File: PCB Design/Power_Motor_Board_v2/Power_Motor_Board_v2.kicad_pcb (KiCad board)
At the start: 2 copper layers, 96 x 94.3 mm, 38 parts, among them IC1 DRV8251ADDAR, IC3 DRV8251ADDAR, IC4 AP63205WU-7, J1 691137710002, J2 691137710002, J2A1 SSW-119-01-T-D, J3 691137710002, J4 Conn_01x06, J5 Conn_01x02_Socket

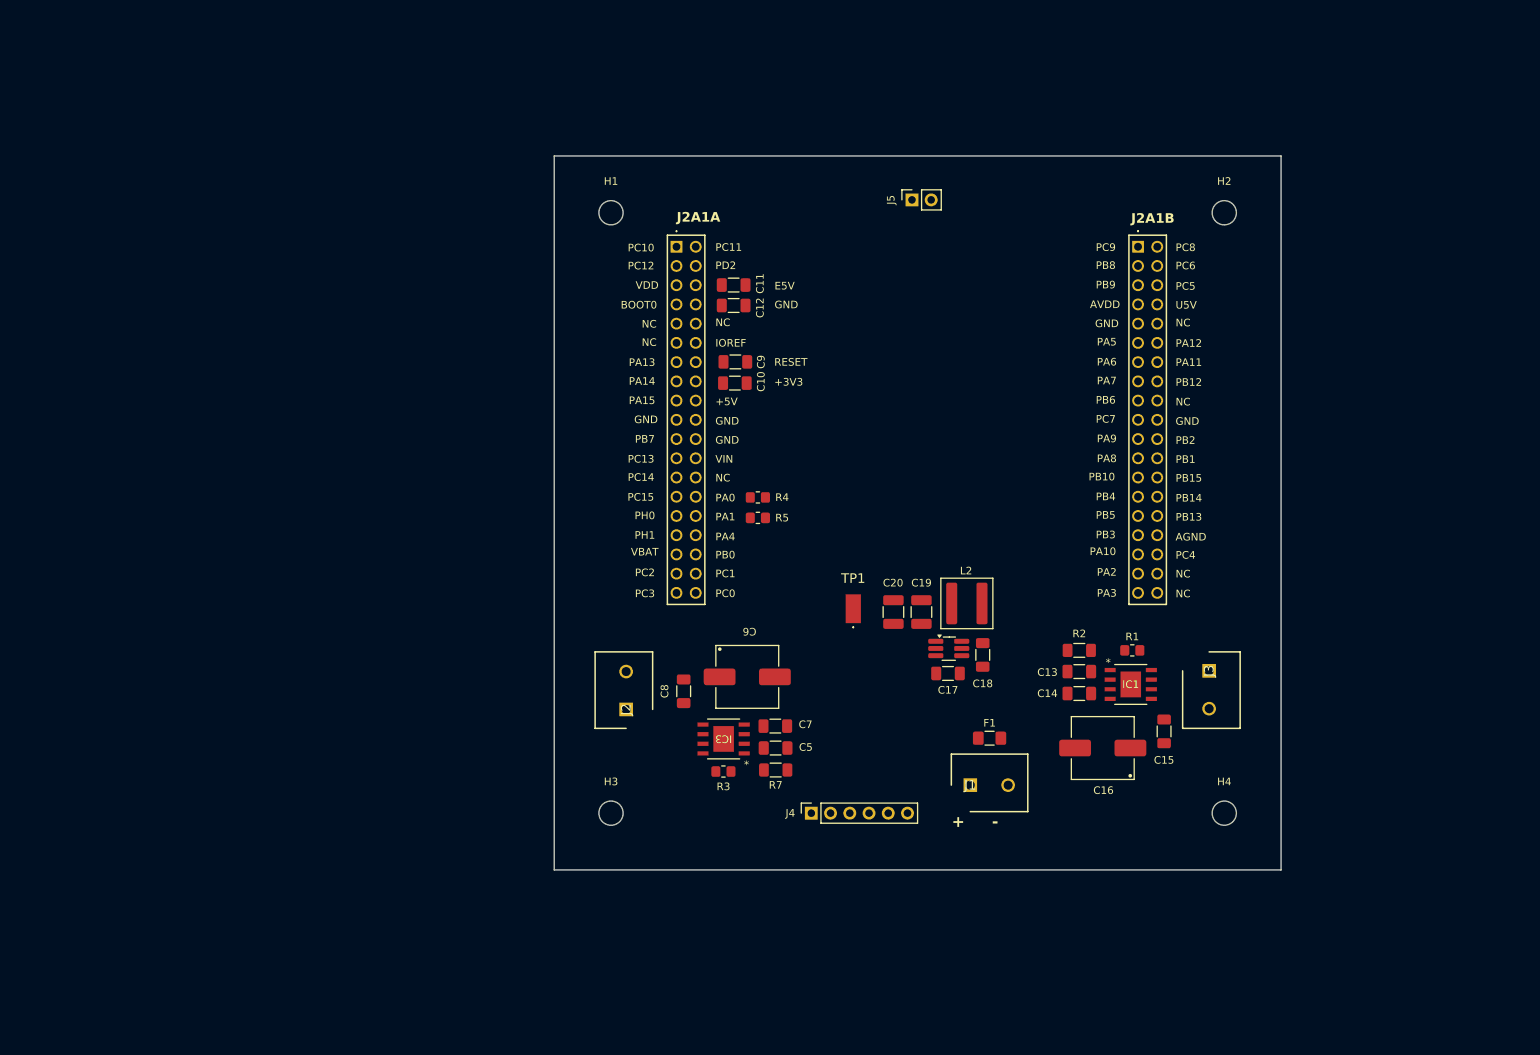
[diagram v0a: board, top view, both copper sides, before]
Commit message: traced out the layout
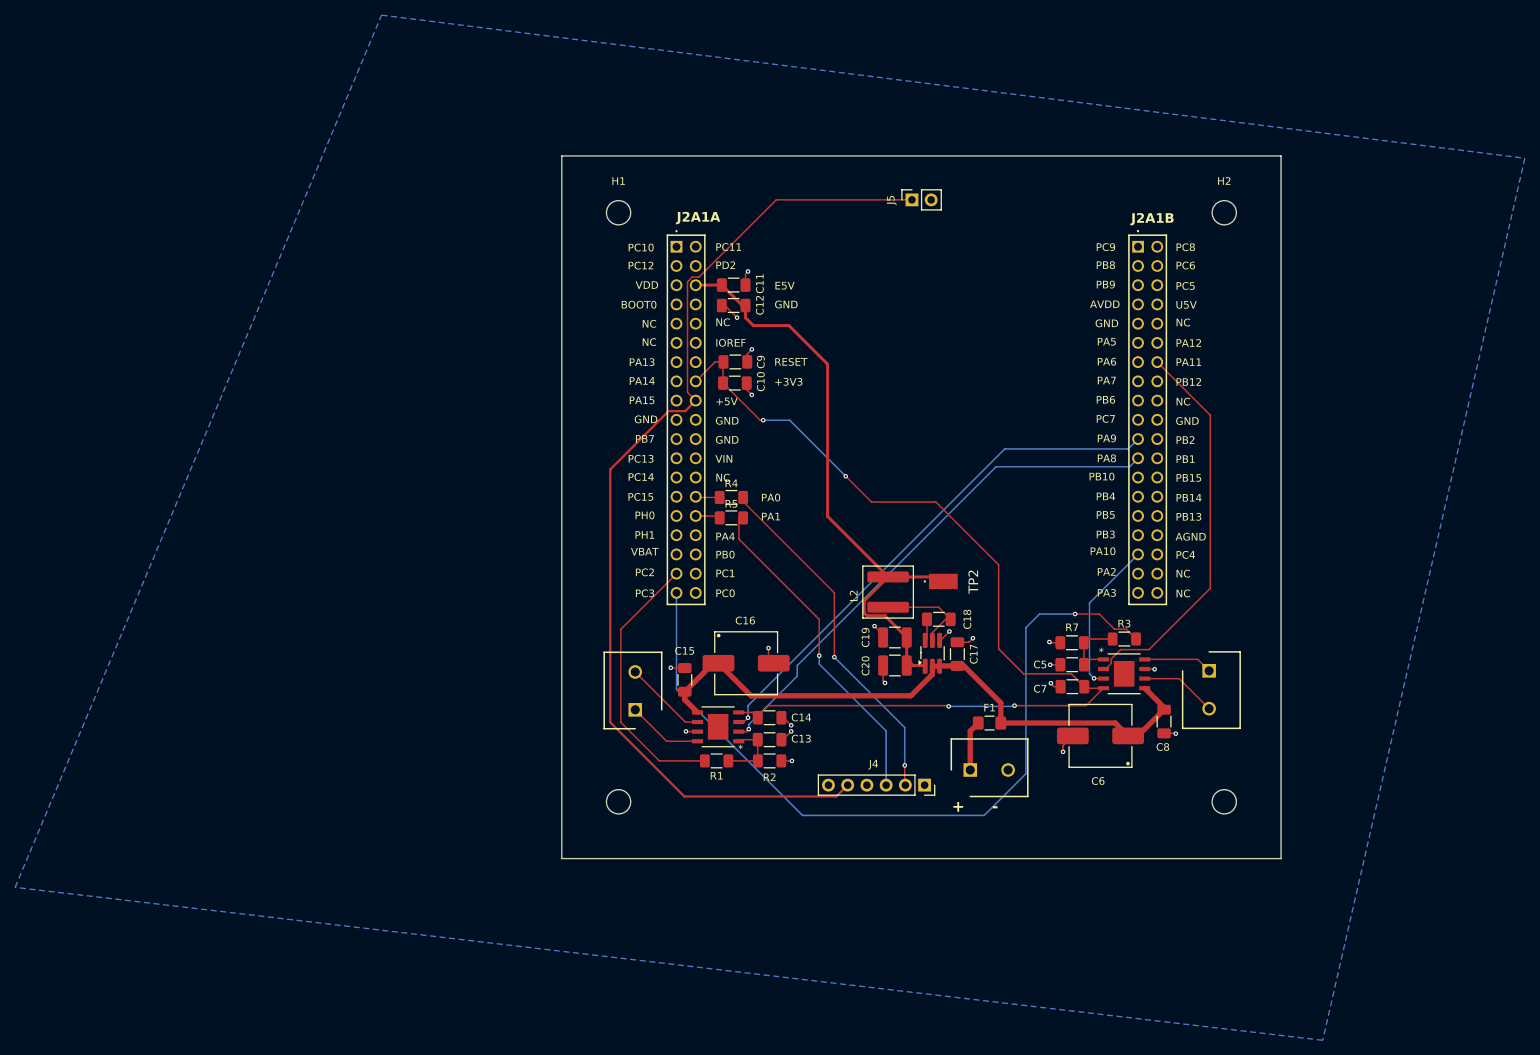
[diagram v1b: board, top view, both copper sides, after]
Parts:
- R1, R3, R4, R5: footprint Resistor_SMD:R_0805_2012Metric_Pad1.20x1.40mm_HandSolder -> Resistor_SMD:R_1206_3216Metric_Pad1.30x1.75mm_HandSolder
- moved J2 77.2 mm to (189.0, 107.2), turned to -90 degrees
- moved J3 76.0 mm to (113.2, 112.3), turned to 90 degrees
- moved C15 63.7 mm to (119.8, 108.4), turned to 90 degrees
- moved C8 63.6 mm to (183.1, 113.9), turned to -90 degrees
- moved C16 59.7 mm to (122.1, 106.2), turned to 0 degrees
- moved C6 58.7 mm to (180.4, 115.8), turned to 180 degrees
- moved R1 56.8 mm to (124.0, 119.1), turned to 0 degrees
- moved R3 55.8 mm to (177.8, 103.0), turned to 180 degrees
- moved IC1 54.8 mm to (124.2, 114.6), turned to 180 degrees
- moved IC3 53.6 mm to (177.8, 107.6), turned to 0 degrees
- moved R2 43.4 mm to (130.9, 119.1), turned to 0 degrees
- moved R7 42.6 mm to (170.9, 103.5), turned to 180 degrees
- moved C13 41.9 mm to (130.9, 116.3), turned to 0 degrees
- moved C14 41.0 mm to (130.9, 113.4), turned to 0 degrees
- moved C5 40.7 mm to (170.9, 106.4), turned to 180 degrees
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- renumbered TP1 to TP2
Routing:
- net 5V_out: track 0.00 -> 134.8 mm
- net +3V3: track 0.00 -> 131.3 mm, vias 0 -> 4
- net /I_MTR2: track 0.00 -> 104.3 mm, vias 0 -> 1
- net +Vbatt: track 0.00 -> 83.0 mm
- net +5V: track 0.00 -> 80.9 mm
- net /IN1_MTR1: track 0.00 -> 69.2 mm, vias 0 -> 1
- net /IN2-MTR1: track 0.00 -> 68.9 mm, vias 0 -> 1
- net /IN2_MTR2: track 0.00 -> 51.6 mm
- net Net-(J4-Pin_2): track 0.00 -> 47.1 mm, vias 0 -> 2
- net Net-(J4-Pin_3): track 0.00 -> 43.4 mm, vias 0 -> 1
- net GND: track 0.00 -> 37.3 mm, vias 0 -> 20
- net /I_MTR1: track 0.00 -> 36.4 mm
- net /IN1_MTR2: track 0.00 -> 20.5 mm, vias 0 -> 1
- net Net-(IC4-SW): track 0.00 -> 13.1 mm
- net /+OUT_1: track 0.00 -> 11.0 mm
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- added copper zone on B.Cu, net GND
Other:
- board size 96 x 94.3 mm -> 95 x 92.8 mm

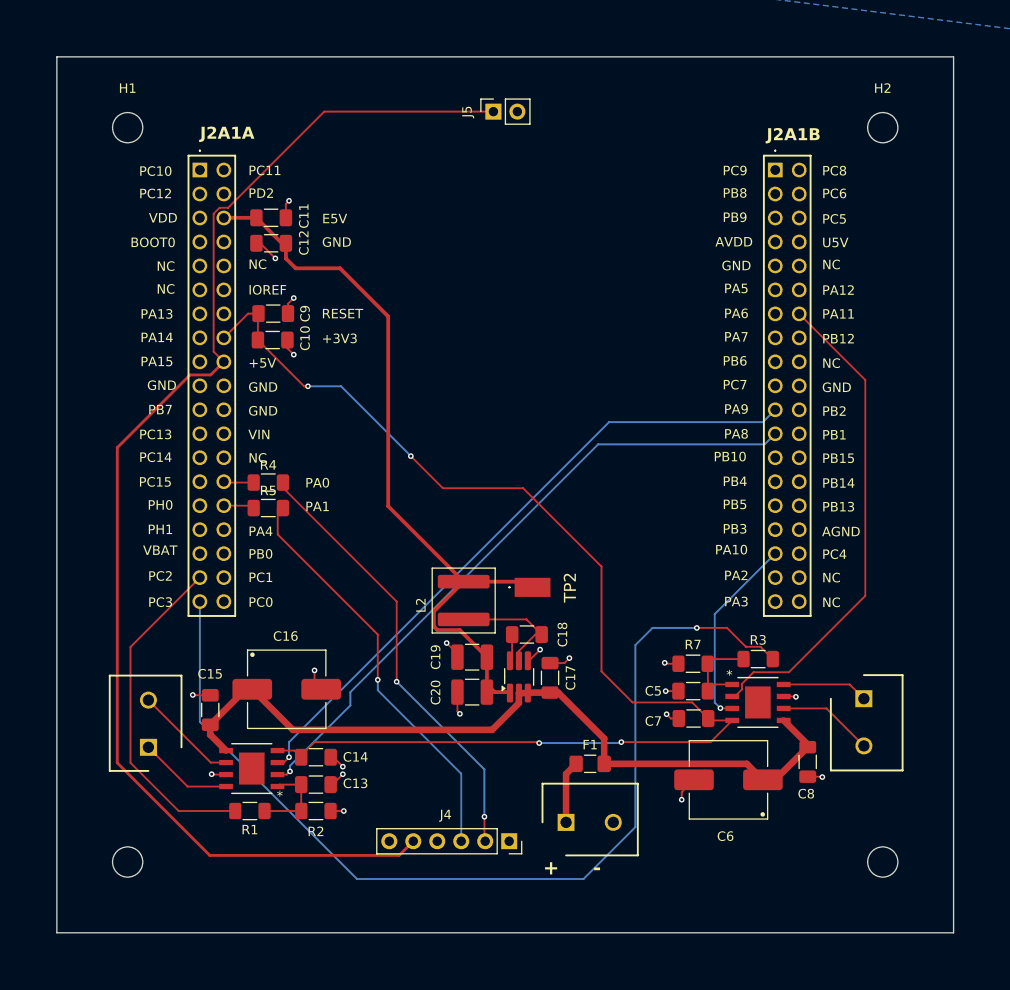
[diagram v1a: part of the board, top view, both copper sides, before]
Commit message: changed to v2 main board
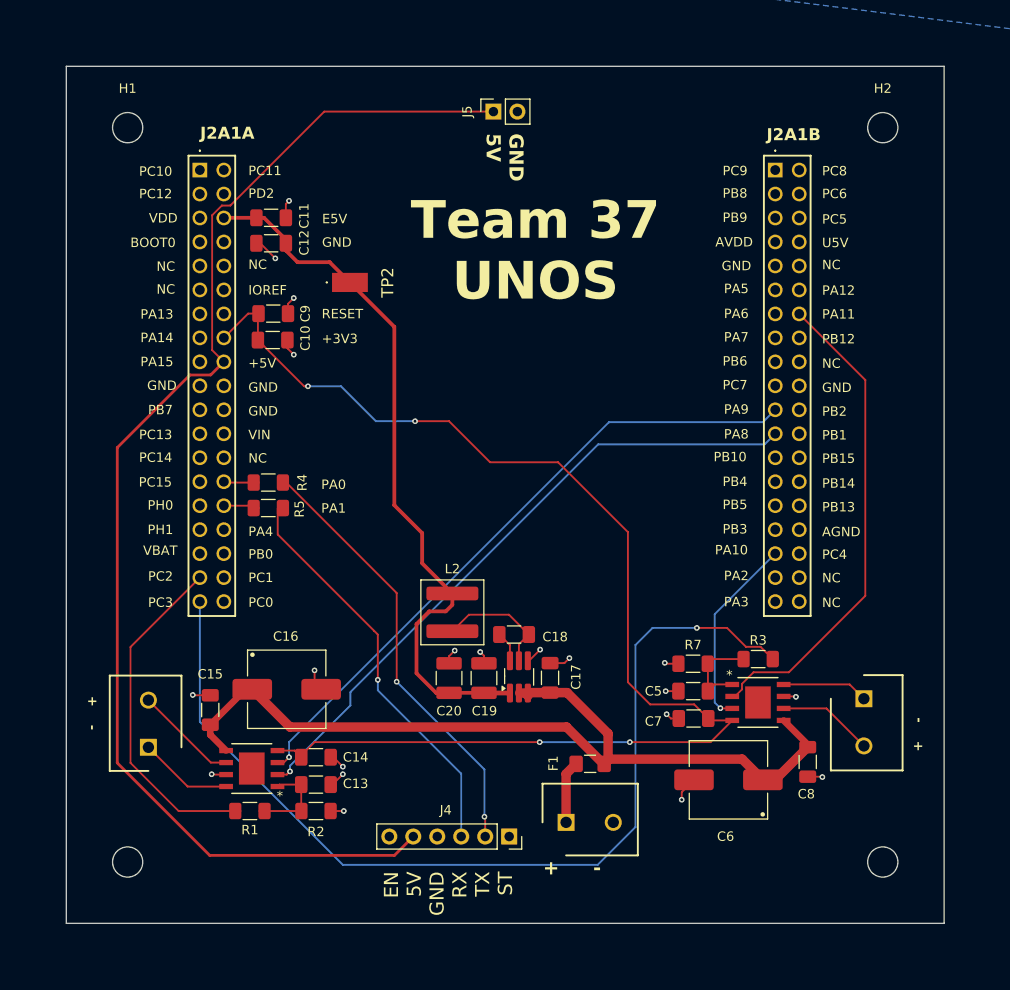
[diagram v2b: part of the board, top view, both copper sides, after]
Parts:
- added G***: LOGO, LOGO, F.Cu at (150.7, 57.7)
- moved TP2 37.7 mm to (134.6, 63.1)
- moved C20 2.87 mm to (145.1, 105.0), turned to -90 degrees
- moved C19 2.54 mm to (148.8, 105.0), turned to -90 degrees
- moved L2 1.73 mm to (145.4, 98.0)
- moved C18 1.36 mm to (151.9, 100.4)
- moved J4 0.50 mm to (151.4, 121.8)
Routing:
- net +Vbatt: track 83.0 -> 94.2 mm
- net +5V: track 80.9 -> 77.2 mm
- net +3V3: track 131.3 -> 134.0 mm
- net GND: track 37.3 -> 35.9 mm
- net /I_MTR2: track 104.3 -> 103.1 mm
- net Net-(IC4-BST): track 2.88 -> 3.58 mm
- net Net-(J4-Pin_2): track 47.1 -> 47.6 mm
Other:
- board size 95 x 92.8 mm -> 93 x 90.8 mm
- board text added: "EN 5V GND RX TX ST"
- board text added: "GND 5V"
- board text added: "Team 37 UNOS"
- board text added: "amazingamy"
- board text added: "freddy fazbear"
- board text added: "jujuthepoopoo"
- board text added: "lean masheen"
- board text added: "whatdahaleeberry"
